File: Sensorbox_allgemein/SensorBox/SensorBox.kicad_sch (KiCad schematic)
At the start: 26 parts, among them SW1 SW_SPST, U1 BME280, U2 PS1-O3-100, U3 Beetle ESP32-C6, U4 MC33063AD, U6 MAX31855EASA, U8 HPP845E131R5

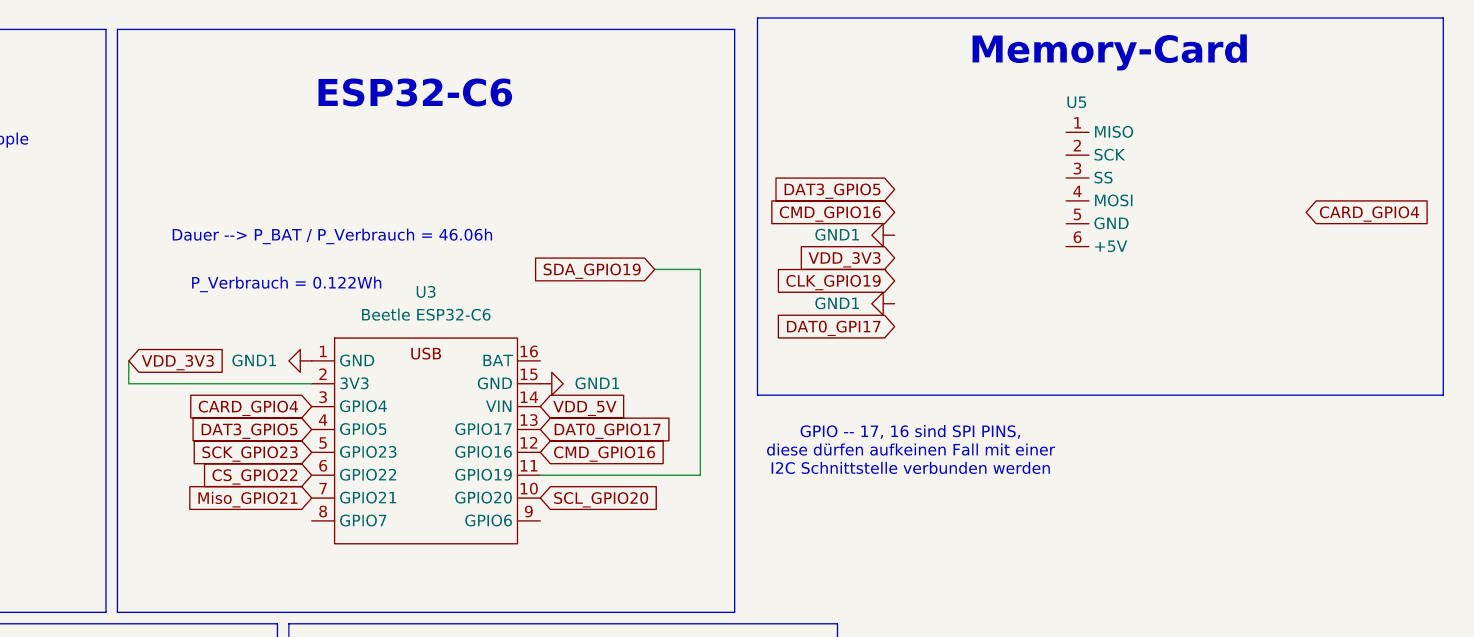
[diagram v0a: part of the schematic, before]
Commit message: Test
.
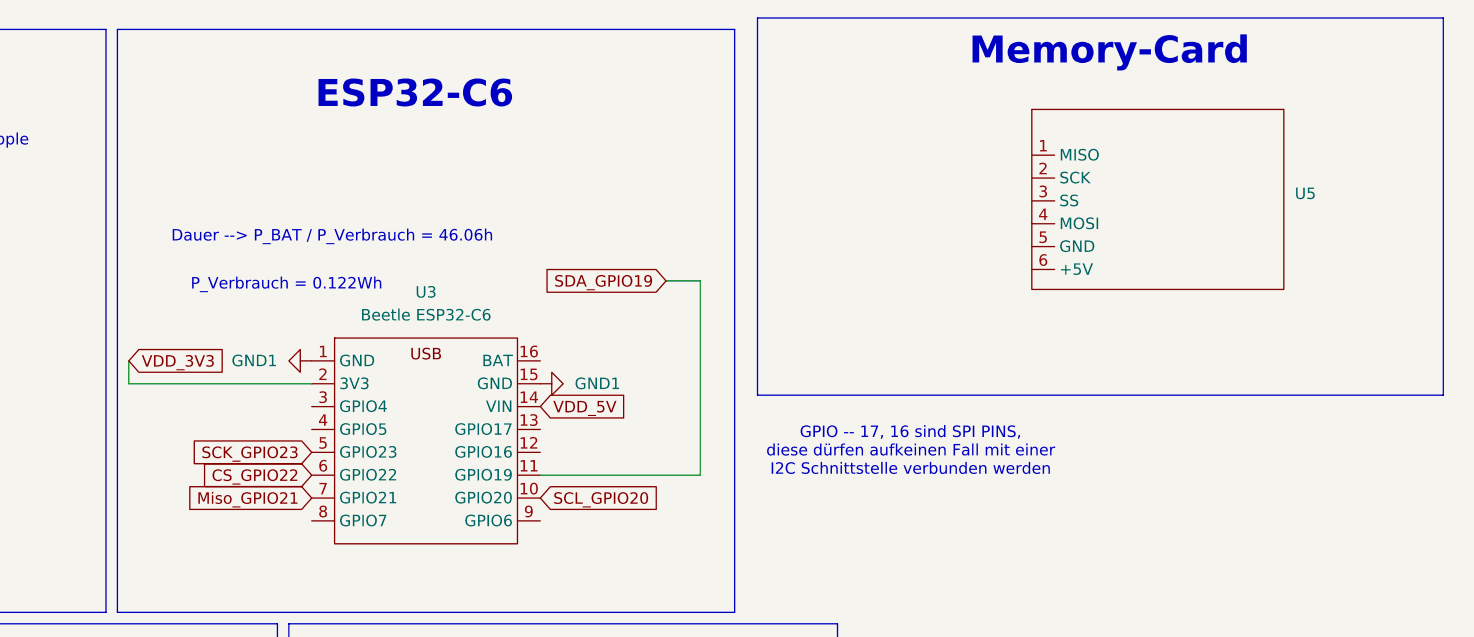
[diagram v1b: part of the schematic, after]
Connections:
- net CARD_GPIO4: no longer names the net of U3.3 (GPIO4)
- net CMD_GPIO16: no longer names the net of U3.12 (GPIO16)
- net DAT0_GPIO17: no longer names the net of U3.13 (GPIO17)
- net DAT3_GPIO5: no longer names the net of U3.4 (GPIO5)
